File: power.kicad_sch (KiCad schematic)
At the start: 30 parts

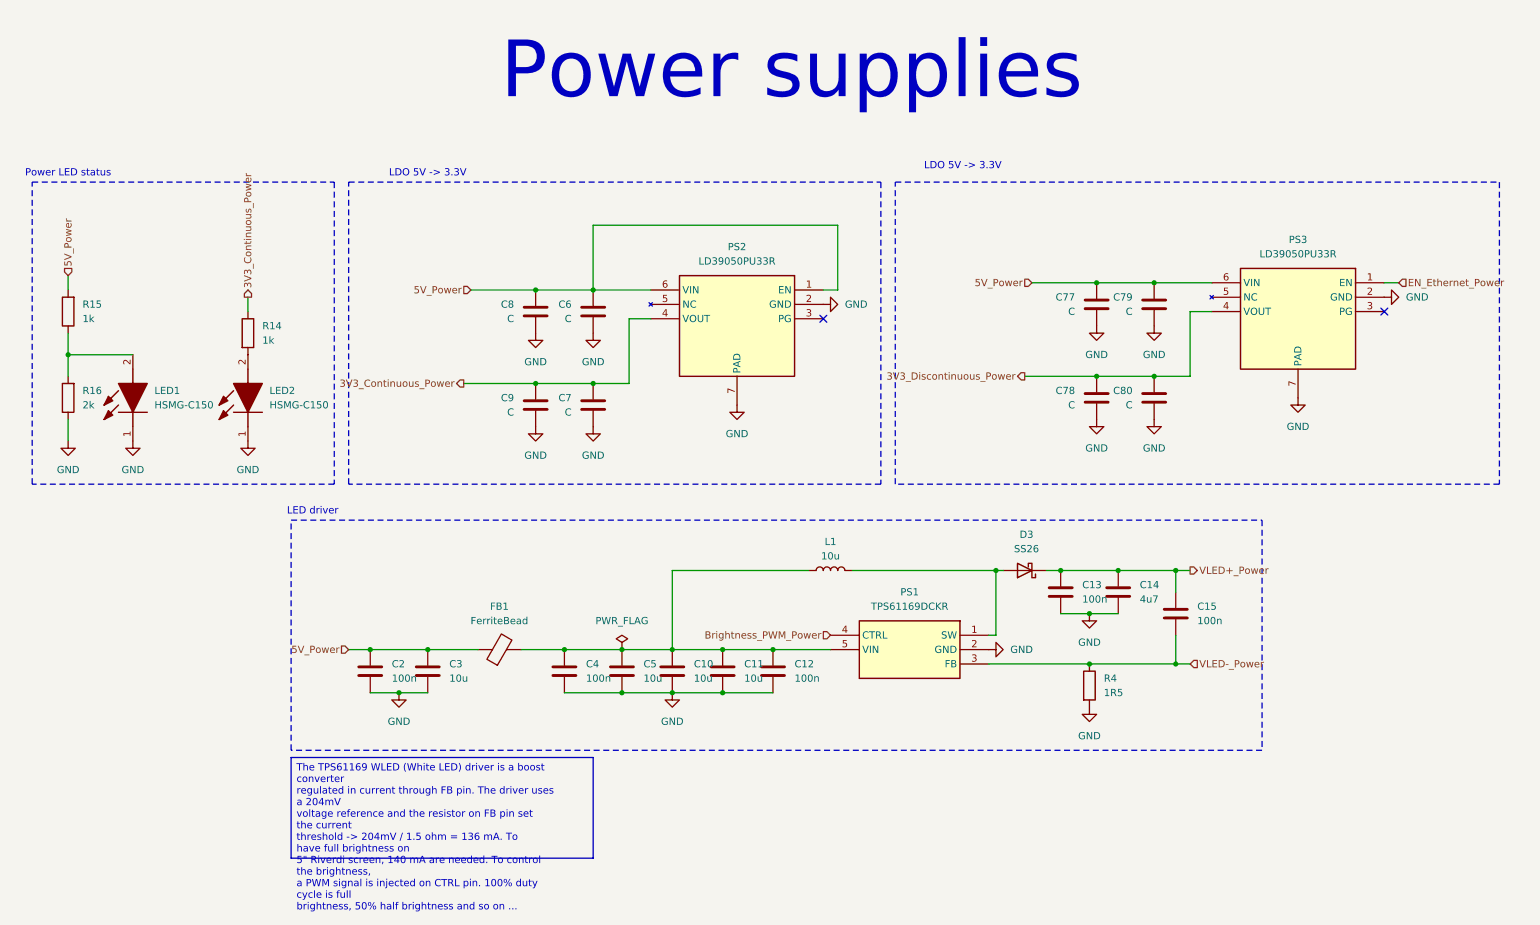
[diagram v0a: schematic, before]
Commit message: Continue schematic review
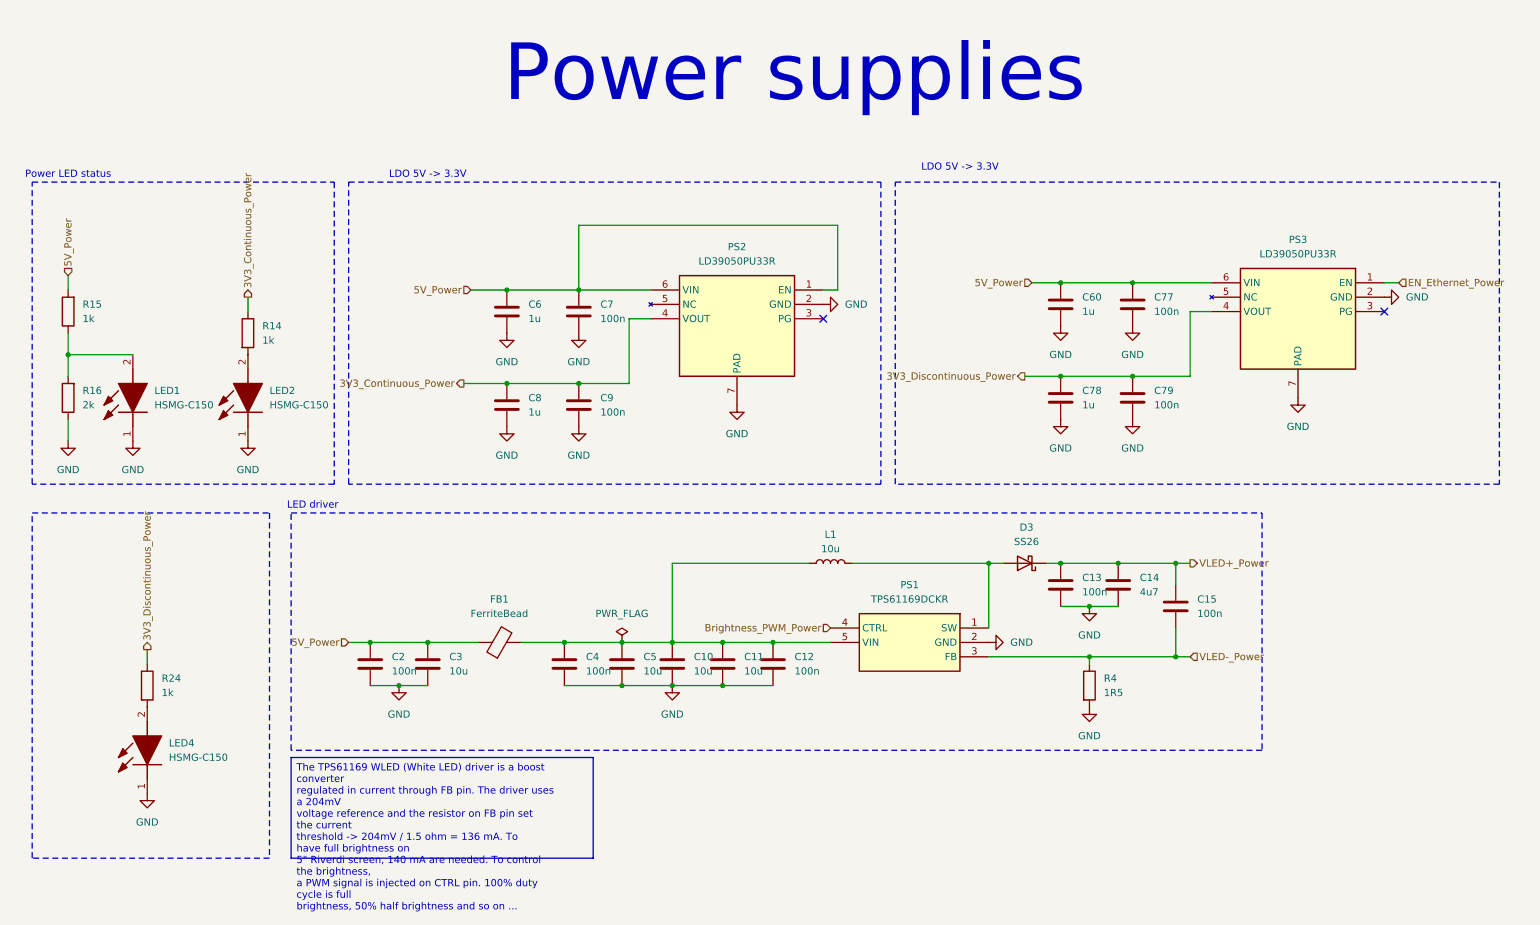
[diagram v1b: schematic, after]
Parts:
- removed C80: C, Capacitor_SMD:C_0603_1608Metric_Pad1.08x0.95mm_HandSolder, symbol Device:C
- added C60: 1u, symbol Device:C
- added LED4: HSMG-C150, weather-station-poc-fp:LEDC3216X120N, symbol weather-station-poc-sym:HSMG-C150
- added R24: 1k, symbol Device:R
- C6, C78, C8: value C -> 1u; footprint Capacitor_SMD:C_0603_1608Metric_Pad1.08x0.95mm_HandSolder -> (none)
- C7, C77, C79, C9: value C -> 100n; footprint Capacitor_SMD:C_0603_1608Metric_Pad1.08x0.95mm_HandSolder -> (none)
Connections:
- net 3V3_Continuous_Power: now also C8.1; no longer C7.1
- net 3V3_Discontinuous_Power: now also C79.1, R24.1
- net 5V_Power: now also C7.1, C60.1; no longer C79.1, C8.1
- net GND: now also C60.2, LED4.1 (K)
- new net: LED4.2 (A), R24.2
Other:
- moved on the sheet: C10, C11, C12, C13, C14, C15, C2, C3, C4, C5, D3, FB1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
